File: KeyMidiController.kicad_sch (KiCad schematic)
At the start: 2 parts, among them U1 HEF4051B, U2 HEF4051B

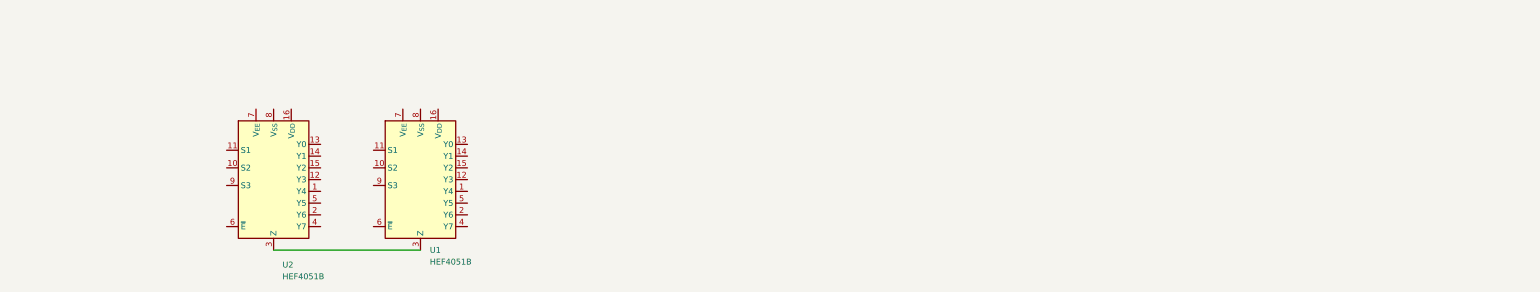
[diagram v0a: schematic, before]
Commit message: Finally documenting the PCB
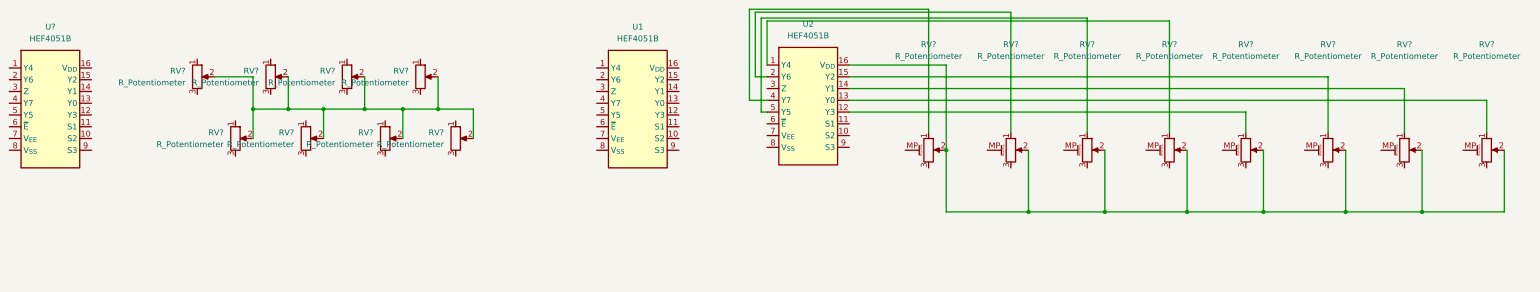
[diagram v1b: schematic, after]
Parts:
- removed U2: HEF4051B, symbol Midi_Keyboard:HEF4051B
- added RV? (x8): R_Potentiometer, symbol Device:R_Potentiometer
- added RV? (x7): R_Potentiometer, Potentiometer_THT:Potentiometer_Bourns_PTA3043_Single_Slide, symbol Device:R_Potentiometer_MountingPin
- added RV?: R_Potentiometer, symbol Device:R_Potentiometer_MountingPin
- added U2, U?: HEF4051B, symbol Armaan_Library:HEF4051B
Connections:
- new net: RV?.2, RV?.2, RV?.2, RV?.2, RV?.2, RV?.2, RV?.2, RV?.2
- new net: RV?.1, U2.15 (Y2)
- new net: RV?.2, RV?.2, RV?.2, RV?.2, RV?.2, RV?.2, RV?.2, RV?.2, U2.16 (V_{DD})
- new net: RV?.1, U2.1 (Y4)
- new net: RV?.1, U2.13 (Y0)
- new net: RV?.1, U2.14 (Y1)
- new net: RV?.1, U2.5 (Y5)
- new net: RV?.1, U2.12 (Y3)
- new net: RV?.1, U2.2 (Y6)
- new net: RV?.1, U2.4 (Y7)

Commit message: Mass Update
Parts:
- removed RV? (x7): R_Potentiometer, Potentiometer_THT:Potentiometer_Bourns_PTA3043_Single_Slide, symbol Device:R_Potentiometer_MountingPin
- removed RV?: R_Potentiometer, symbol Device:R_Potentiometer_MountingPin
- added J?: DIN41612_02x08_AC_EvenPins, symbol Connector:DIN41612_02x08_AC_EvenPins
- added LINEAR, ROTARY, U?: HEF4051B, symbol Armaan_Library:HEF4051B
- added RV1, RV2, RV3, RV4, RV5, RV6, RV7, RV8: R_Potentiometer, symbol Device:R_Potentiometer
- added RV10, RV11, RV12, RV13, RV14, RV15, RV16, RV9, RV? (x8): R_Potentiometer, Potentiometer_THT:Potentiometer_Bourns_PTA3043_Single_Slide, symbol Device:R_Potentiometer_MountingPin
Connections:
- net at RV?.1: now also RV?.1, RV?.1, RV?.1, RV?.1, RV?.1, RV?.1, RV?.1, U1.7 (V_{EE}), U1.8 (V_{SS}), J?.Red (Pin_c6)
- net at RV?.3: now also RV?.3, RV?.3, RV?.3, RV?.3, RV?.3, RV?.3, RV?.3, U1.16 (V_{DD}), U2.16 (V_{DD}), U?.16 (V_{DD}), J?.Black, RV?.3, RV?.3, RV?.3, RV?.3, RV?.3, RV?.3, RV?.3, RV?.3
- net at U2.15 (Y2): now also RV?.2
- net at U2.1 (Y4): now also RV?.2
- net at U2.13 (Y0): now also RV?.2
- net at U?.10 (S2): now also U1.6 (~{E}), J?.Purple (Pin_c16)
- net at U?.11 (S1): now also U2.6 (~{E}), J?.Blue (Pin_c14)
- net at U?.3 (Z): now also U1.3 (Z), U2.3 (Z), J?.Brown (Pin_c4)
- net at U2.14 (Y1): now also RV?.2
- net at U2.5 (Y5): now also RV?.2
- net at U2.12 (Y3): now also RV?.2
- net at U2.10 (S2): now also U1.10 (S2), J?.Yellow (Pin_c10)
- net at U2.11 (S1): now also U1.11 (S1), J?.Orange (Pin_c8)
- net at U2.2 (Y6): now also RV?.2
- net at U2.4 (Y7): now also RV?.2
- net at U2.7 (V_{EE}): now also U2.8 (V_{SS})
- net at U2.9 (S3): now also U1.9 (S3), J?.Green (Pin_c12)
- net at U1.1 (Y4): now also RV?.2
- net at U1.12 (Y3): now also RV?.2
- net at U1.13 (Y0): now also RV?.2
- net at U1.14 (Y1): now also RV?.2
- net at U1.15 (Y2): now also RV?.2
- net at U1.2 (Y6): now also RV?.2
- net at U1.4 (Y7): now also RV?.2
- net at U1.5 (Y5): now also RV?.2
- new net: RV13.3, RV14.3, RV15.3, RV16.3
- new net: LINEAR.6 (~{E}), U?.11 (S1)
- new net: LINEAR.7 (V_{EE}), LINEAR.8 (V_{SS})
- new net: RV?.1, RV?.1, RV?.1, RV?.1, RV?.1, RV?.1, RV?.1, RV?.1
- new net: ROTARY.6 (~{E}), U?.10 (S2)
- new net: ROTARY.7 (V_{EE}), ROTARY.8 (V_{SS})
- new net: U?.7 (V_{EE}), U?.8 (V_{SS})
- new net Black: LINEAR.16 (V_{DD}), ROTARY.16 (V_{DD}), RV1.1, RV1.3, RV10.3, RV11.3, RV12.3, RV2.1, RV2.3, RV3.1, RV3.3, RV4.1, RV4.3, RV5.1, RV5.3, RV6.1, RV6.3, RV7.1, RV7.3, RV8.1, RV8.3, RV9.3, U?.16 (V_{DD})
- new net Green: LINEAR.9 (S3), ROTARY.9 (S3)
- new net Orange: LINEAR.11 (S1), ROTARY.11 (S1)
- new net Red: RV10.1, RV11.1, RV12.1, RV13.1, RV14.1, RV15.1, RV16.1, RV9.1
- new net Y0: RV12.2, RV4.2
- new net Y1: RV11.2, RV3.2
- new net Y2: RV10.2, RV2.2
- new net Y3: RV1.2, RV9.2
- new net Y4: RV16.2, RV8.2
- new net Y5: RV15.2, RV7.2
- new net Y6: RV14.2, RV6.2
- new net Y7: RV13.2, RV5.2
- new net Yellow: LINEAR.10 (S2), ROTARY.10 (S2)
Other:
- added sheet Mux (untitled.kicad_sch)
- moved on the sheet: RV?, U1, U2, U?
